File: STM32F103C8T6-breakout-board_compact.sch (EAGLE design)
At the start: 37 parts, among them J3 AVX_6-PIN_009159006061916, J4 CORTEX_DEBUG_PTH, J5 10118194-0001LF, U1 STM32F103C8T6, U2 CJT1117-3.3-SOT223

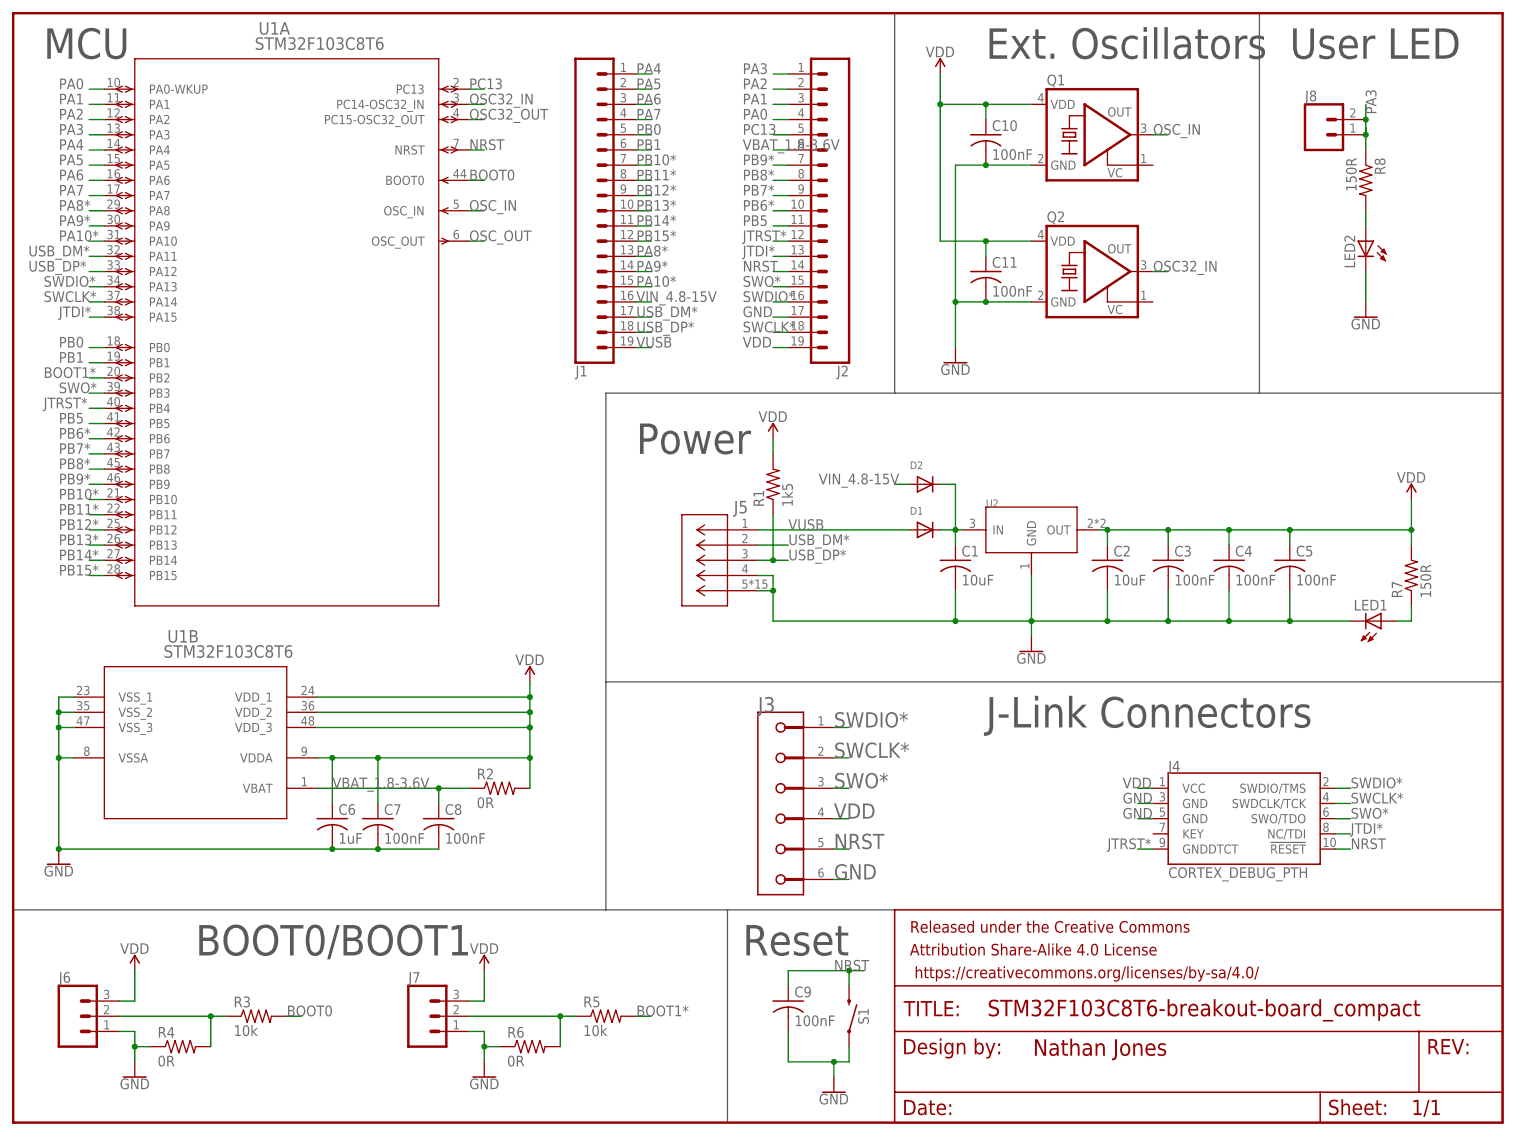
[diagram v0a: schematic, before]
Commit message: Updated files.
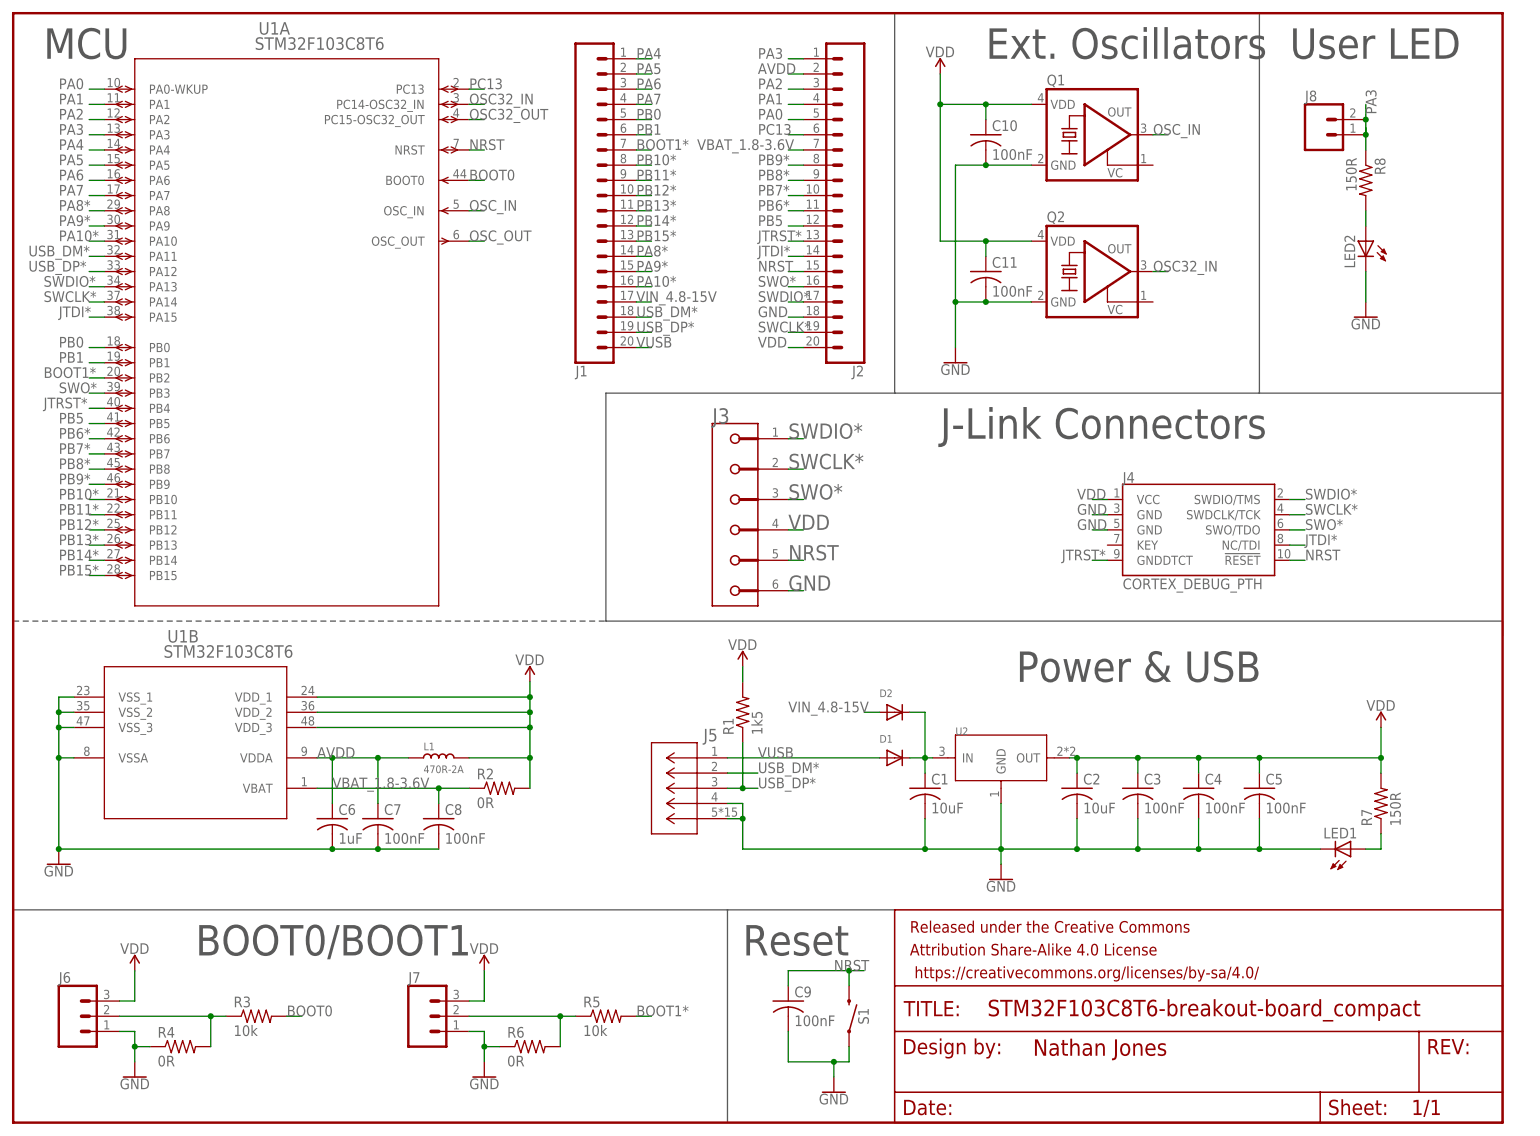
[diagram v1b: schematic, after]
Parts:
- added L1: 470R-2A, OPL_Ferrite_and_Magnetic_Bead:SMD-FERRITE-BEAD-470R-2A(0805)'0805'
- J1, J2: device SparkFun-Connectors:CONN_191X19_NO_SILK -> SparkFun-Connectors:CONN_20NOSILK
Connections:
- new net AVDD: C6.1, C7.1, J2.2, L1.1, U1B.VDDA
- net BOOT1*: now also J1.7
- net GND: now also J2.18; no longer J2.17
- net JTDI*: now also J2.14; no longer J2.13
- net JTRST*: now also J2.13; no longer J2.12
- net NRST: now also J2.15; no longer J2.14
- net PA0: now also J2.5; no longer J2.4
- net PA1: now also J2.4; no longer J2.3
- net PA10*: now also J1.16; no longer J1.15
- net PA2: now also J2.3; no longer J2.2
- net PA8*: now also J1.14; no longer J1.13
- net PA9*: now also J1.15; no longer J1.14
- net PB10*: now also J1.8; no longer J1.7
- net PB11*: now also J1.9; no longer J1.8
- net PB12*: now also J1.10; no longer J1.9
- net PB13*: now also J1.11; no longer J1.10
- net PB14*: now also J1.12; no longer J1.11
- net PB15*: now also J1.13; no longer J1.12
- net PB5: now also J2.12; no longer J2.11
- net PB6*: now also J2.11; no longer J2.10
- net PB7*: now also J2.10; no longer J2.9
- net PB8*: now also J2.9; no longer J2.8
- net PB9*: now also J2.8; no longer J2.7
- net PC13: now also J2.6; no longer J2.5
- net SWCLK*: now also J2.19; no longer J2.18
- net SWDIO*: now also J2.17; no longer J2.16
- net SWO*: now also J2.16; no longer J2.15
- net USB_DM*: now also J1.18; no longer J1.17
- net USB_DP*: now also J1.19; no longer J1.18
- net VBAT_1.8-3.6V: now also J2.7; no longer J2.6
- net VDD: now also J2.20, L1.2; no longer C6.1, C7.1, J2.19, U1B.VDDA
- net VIN_4.8-15V: now also J1.17; no longer J1.16
- net VUSB: now also J1.20; no longer J1.19
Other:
- note added: "Power & USB"
- note removed: "Power"
- moved on the sheet: C1, C2, C3, C4, C5, D1, D2, J3, J4, J5, LED1, R1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
